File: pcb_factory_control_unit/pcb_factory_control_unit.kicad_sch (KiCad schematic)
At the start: 46 parts, among them J1 CAN, J2 STDC14, J3 Micro_SD_Card_Det1, SW1 Reset, SW2 Boot, U1 STM32H563VITx, U2 SIT3051TK

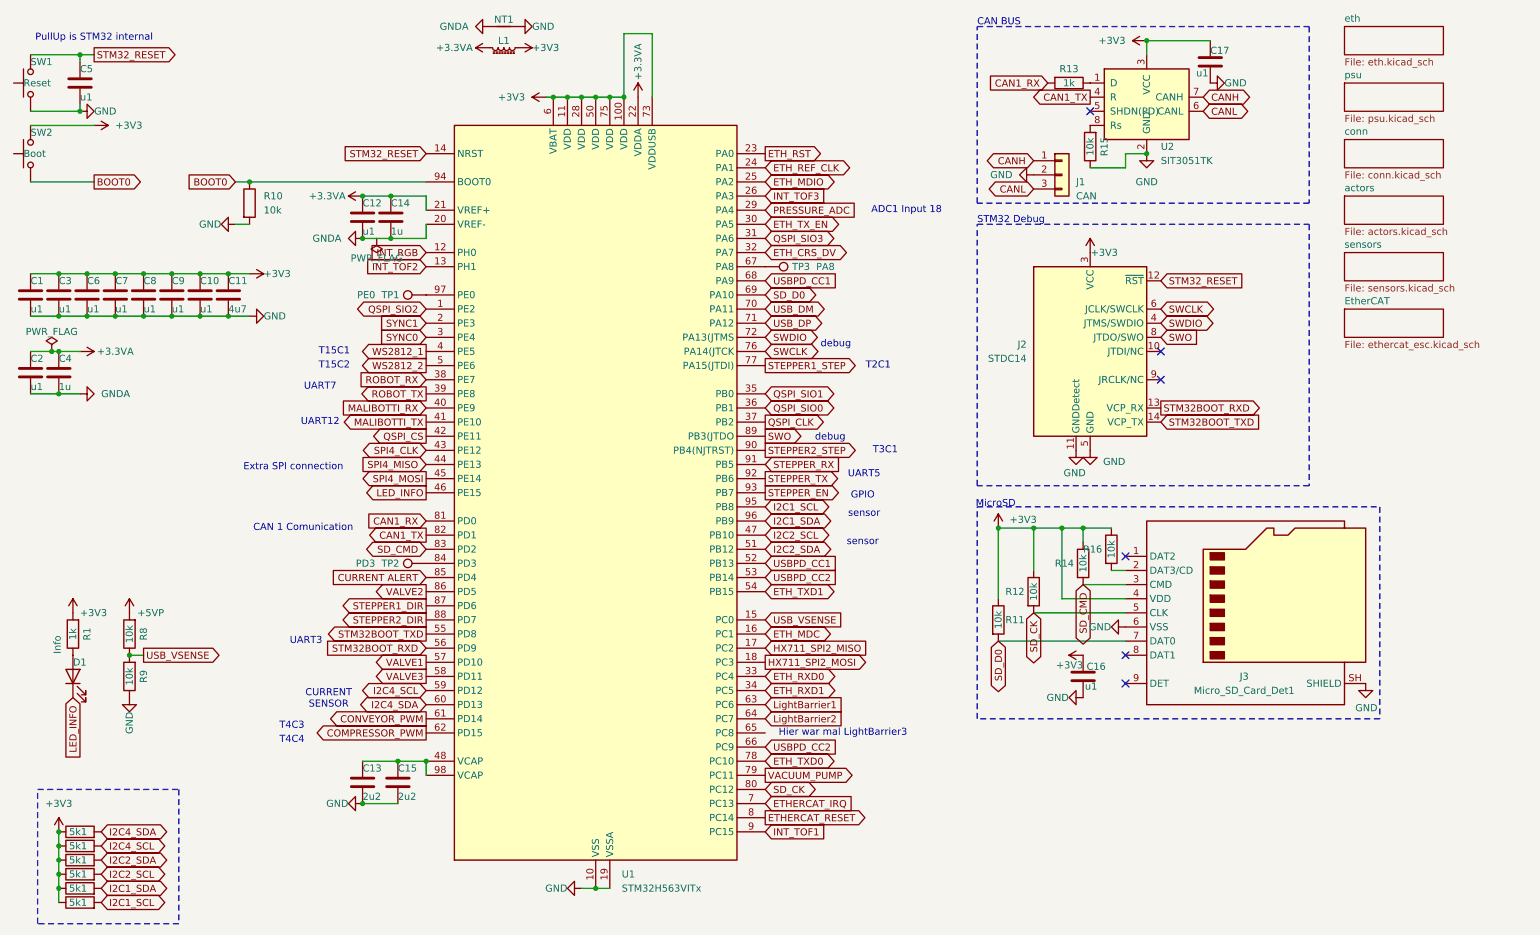
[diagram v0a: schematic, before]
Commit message: WIP PCB
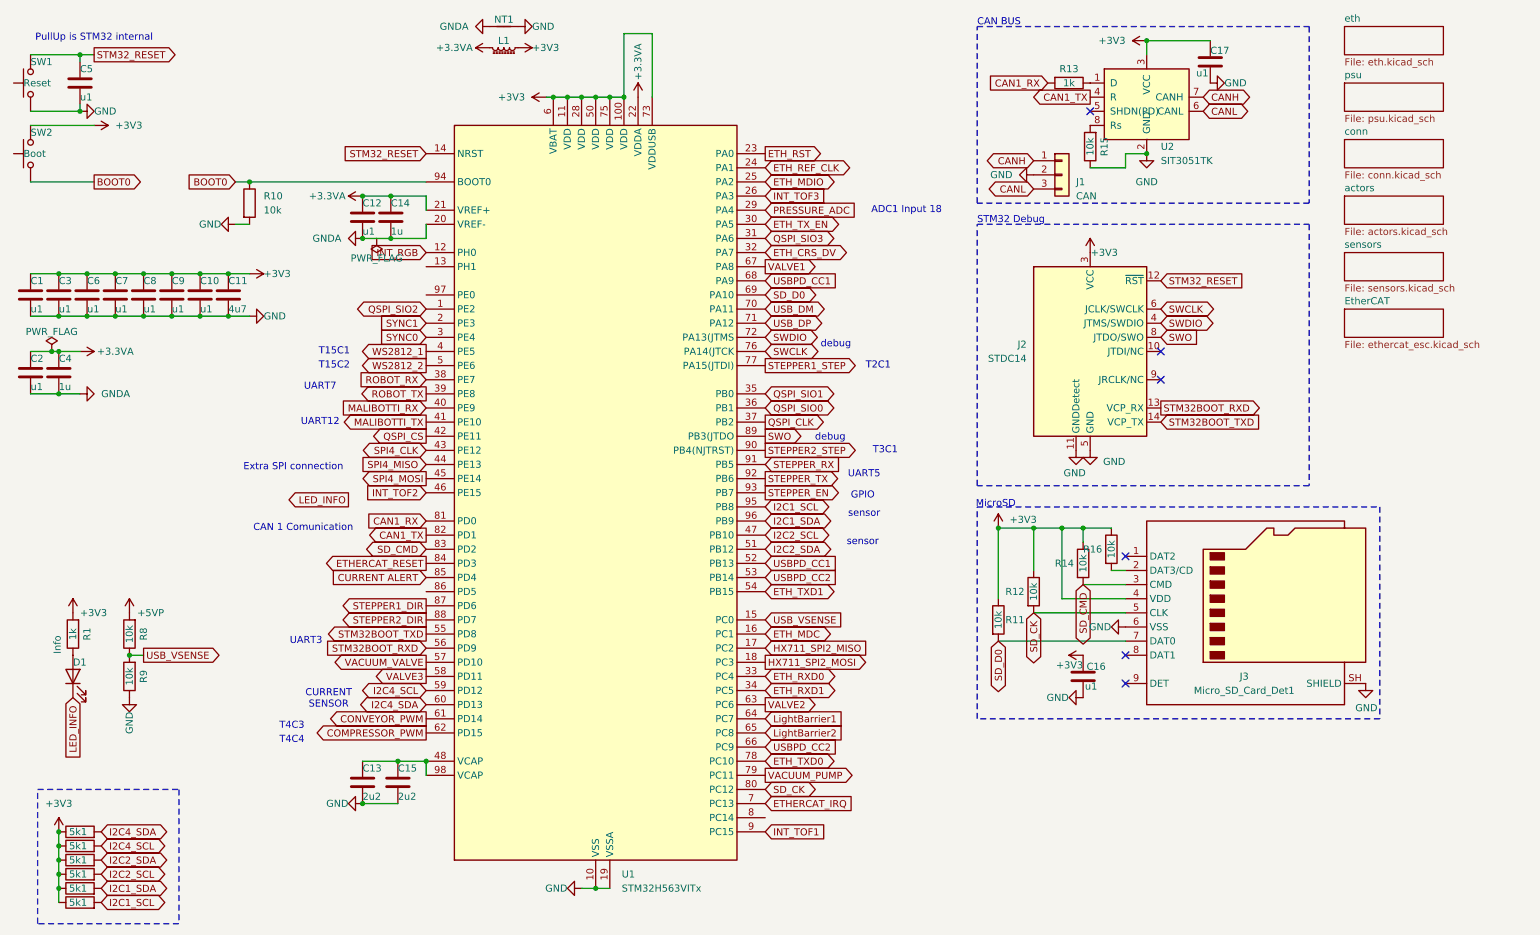
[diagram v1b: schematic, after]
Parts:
- removed TP1: PE0, TestPoint:TestPoint_THTPad_D1.0mm_Drill0.5mm, symbol Connector:TestPoint
- removed TP2: PD3, TestPoint:TestPoint_THTPad_D1.0mm_Drill0.5mm, symbol Connector:TestPoint
- removed TP3: PA8, TestPoint:TestPoint_THTPad_D1.0mm_Drill0.5mm, symbol Connector:TestPoint
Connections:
- net ETHERCAT_RESET: now also U1.84 (PD3); no longer U1.8 (PC14)
- net INT_TOF2: now also U1.46 (PE15); no longer U1.13 (PH1)
- net LED_INFO: no longer U1.46 (PE15)
- net LightBarrier1: now also U1.64 (PC7); no longer U1.63 (PC6)
- net LightBarrier2: now also U1.65 (PC8); no longer U1.64 (PC7)
- net VALVE1: now also U1.67 (PA8); no longer U1.57 (PD10)
- net VALVE2: now also U1.63 (PC6); no longer U1.86 (PD5)
- new net VACUUM_VALVE: U1.57 (PD10)
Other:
- note removed: "Hier war mal LightBarrier3"
